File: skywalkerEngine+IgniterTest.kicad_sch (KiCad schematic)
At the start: 45 parts

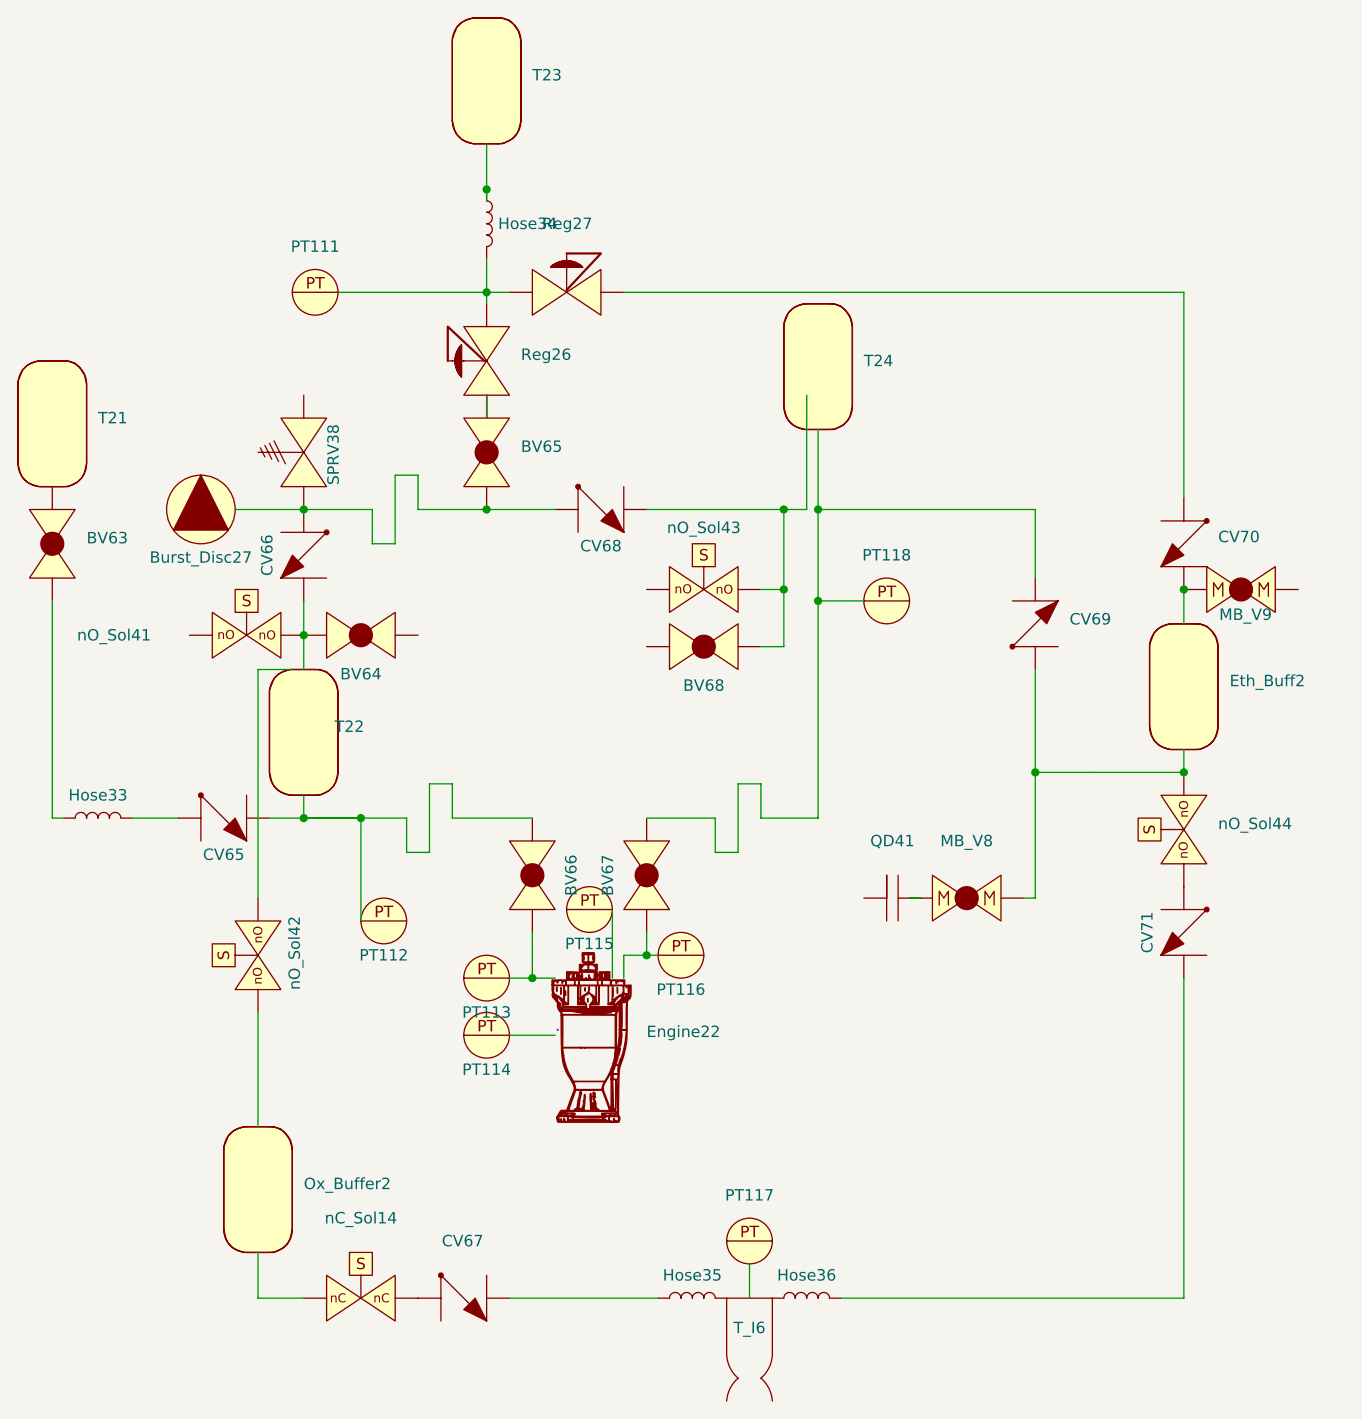
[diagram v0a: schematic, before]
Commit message: j0
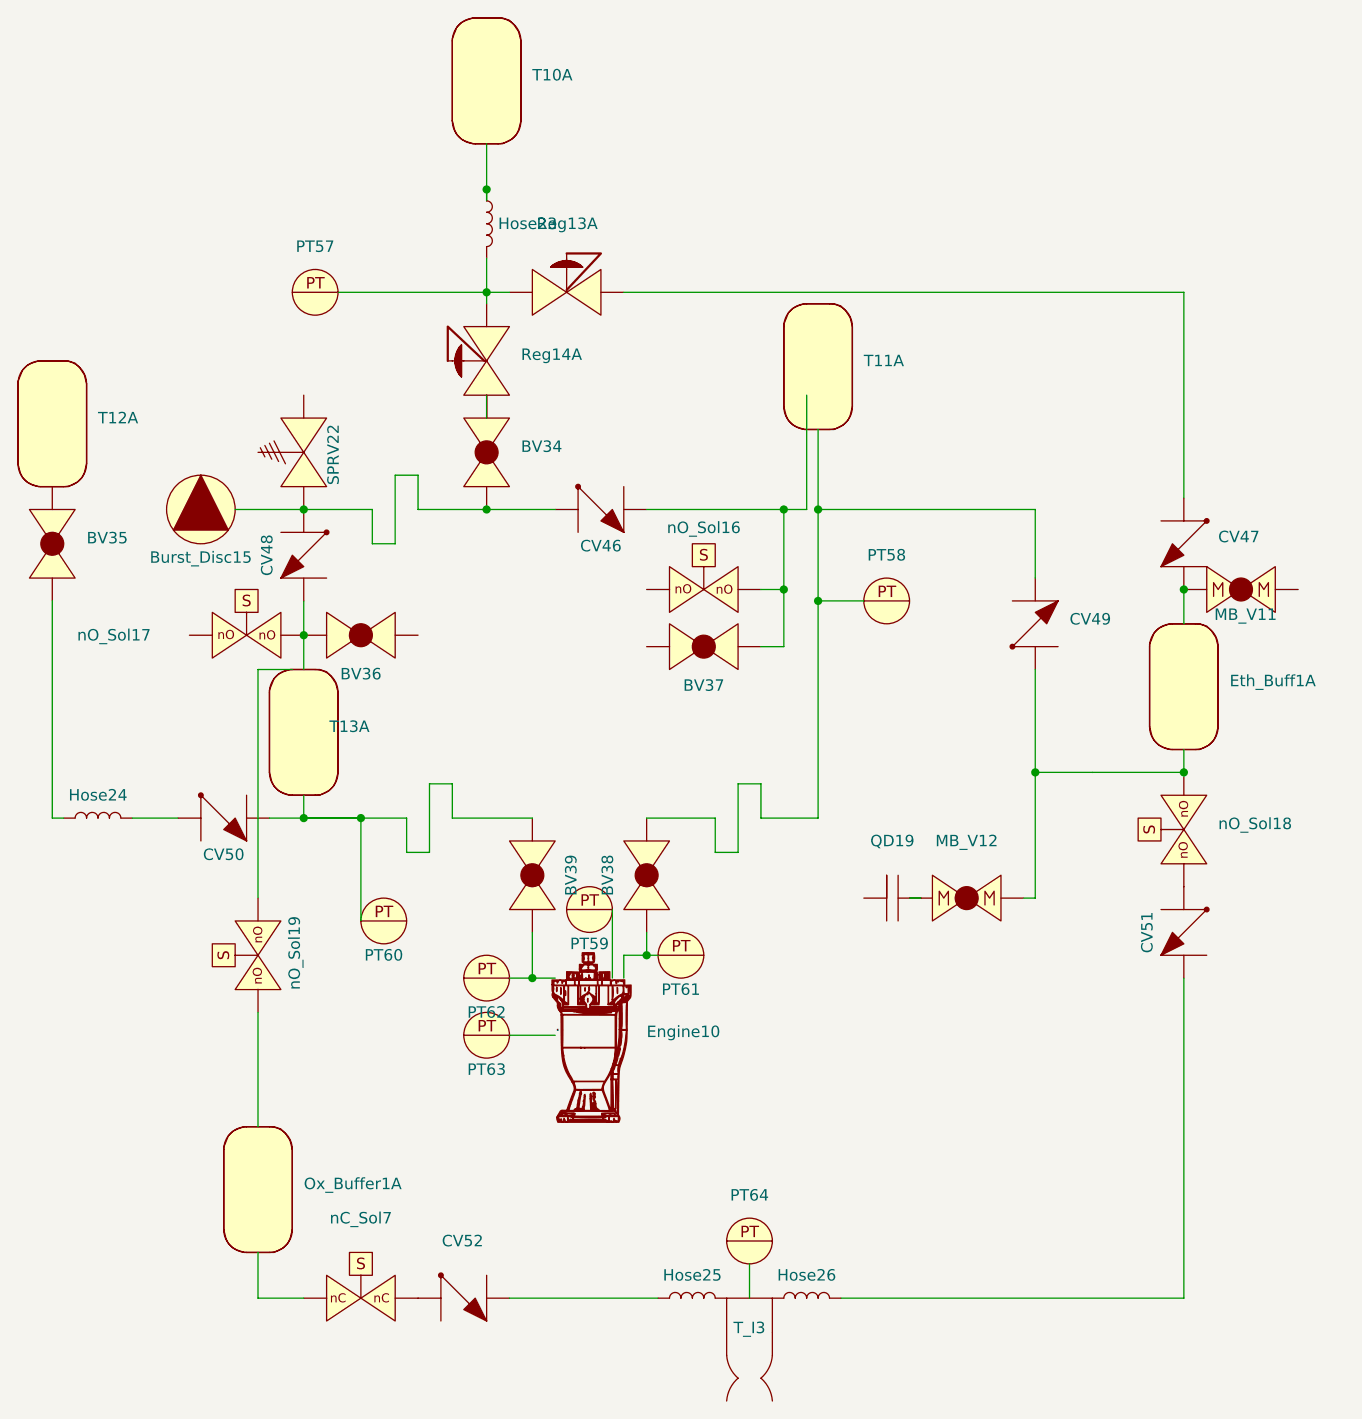
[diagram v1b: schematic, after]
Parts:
- renumbered BV65 to BV34, BV63 to BV35, BV64 to BV36, BV68 to BV37, BV67 to BV38, BV66 to BV39, Burst_Disc27 to Burst_Disc15, CV68 to CV46, CV70 to CV47, CV66 to CV48, CV69 to CV49, CV65 to CV50, CV71 to CV51, CV67 to CV52, Engine22 to Engine10, Eth_Buff2 to Eth_Buff1, Hose34 to Hose23, Hose33 to Hose24, Hose35 to Hose25, Hose36 to Hose26, MB_V9 to MB_V11, MB_V8 to MB_V12, Ox_Buffer2 to Ox_Buffer1, PT111 to PT57, PT118 to PT58, PT115 to PT59, PT112 to PT60, PT116 to PT61, PT113 to PT62, PT114 to PT63, PT117 to PT64, QD41 to QD19, Reg27 to Reg13, Reg26 to Reg14, SPRV38 to SPRV22, T23 to T10, T24 to T11, T21 to T12, T22 to T13, T_I6 to T_I3, nC_Sol14 to nC_Sol7, nO_Sol43 to nO_Sol16, nO_Sol41 to nO_Sol17, nO_Sol44 to nO_Sol18, nO_Sol42 to nO_Sol19
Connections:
- net at Engine10.: now also BV39., PT62.
- net at nC_Sol7.: now also Ox_Buffer1.; no longer CV52.
- net at Ox_Buffer1.: now also nO_Sol19.; no longer nC_Sol7.
- net at T10.: now also Hose23.1
- net at BV36.: now also CV48., T13., nO_Sol17.
- net at T12.: now also BV35.
- net at BV35.: now also Hose24.1; no longer T12.
- net at QD19.: now also MB_V12.
- net at BV37.: now also CV46., nO_Sol16.
- new net: CV49., Eth_Buff1., MB_V12., nO_Sol18.
- new net: BV38., CV49., PT58., T11.
- new net: BV38., Engine10., PT61.
- new net: CV47., Eth_Buff1., MB_V11.
- new net: CV52., nC_Sol7.
- new net: BV39., CV50., PT60., T13.
- new net: BV34., Burst_Disc15., CV46., CV48., SPRV22.
- now unconnected: Burst_Disc15., MB_V11., PT58., PT60., PT61., PT62., SPRV22., T11., nO_Sol16., nO_Sol17.

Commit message: more silwood stuff
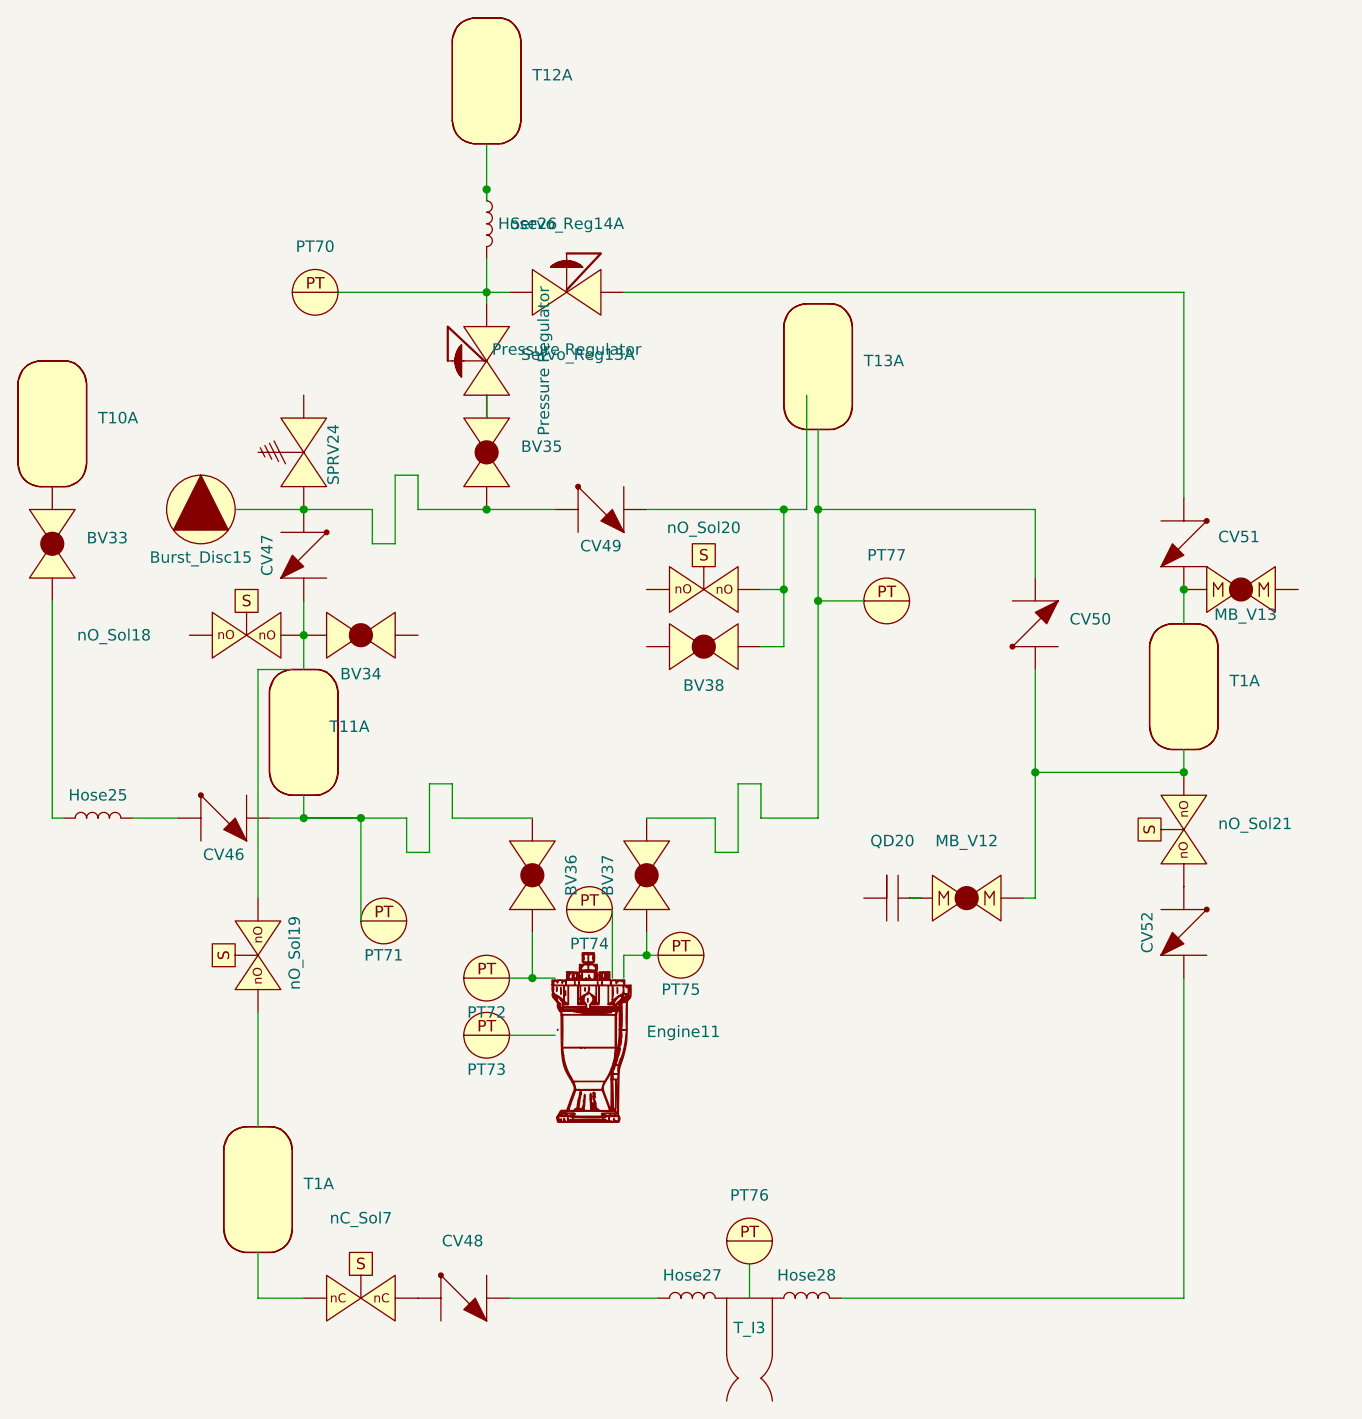
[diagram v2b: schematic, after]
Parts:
- renumbered BV35 to BV33, BV36 to BV34, BV34 to BV35, BV39 to BV36, BV38 to BV37, BV37 to BV38, CV50 to CV46, CV48 to CV47, CV52 to CV48, CV46 to CV49, CV49 to CV50, CV47 to CV51, CV51 to CV52, Engine10 to Engine11, Hose24 to Hose25, Hose23 to Hose26, Hose25 to Hose27, Hose26 to Hose28, MB_V11 to MB_V13, PT57 to PT70, PT60 to PT71, PT62 to PT72, PT63 to PT73, PT59 to PT74, PT61 to PT75, PT64 to PT76, PT58 to PT77, QD19 to QD20, SPRV22 to SPRV24, Reg14 to Servo_Reg13, Reg13 to Servo_Reg14, Eth_Buff1 to T1, Ox_Buffer1 to T1, T12 to T10, T13 to T11, T10 to T12, T11 to T13, nO_Sol17 to nO_Sol18, nO_Sol16 to nO_Sol20, nO_Sol18 to nO_Sol21
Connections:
- net at Engine11.: now also BV36., PT72.
- net at nC_Sol7.: now also T1.; no longer CV48.
- net at T1.: now also nO_Sol19.; no longer nC_Sol7.
- net at T12.: now also Hose26.1
- net at BV34.: now also CV47., T11., nO_Sol18.
- net at T10.: now also BV33.
- net at BV33.: now also Hose25.1; no longer T10.
- net at QD20.: now also MB_V12.
- net at BV38.: now also CV49., nO_Sol20.
- new net: CV50., MB_V12., T1., nO_Sol21.
- new net: BV37., CV50., PT77., T13.
- new net: BV37., Engine11., PT75.
- new net: CV51., MB_V13., T1.
- new net: CV48., nC_Sol7.
- new net: BV36., CV46., PT71., T11.
- new net: BV35., Burst_Disc15., CV47., CV49., SPRV24.
- now unconnected: Burst_Disc15., MB_V13., PT71., PT72., PT75., PT77., SPRV24., T13., nO_Sol18., nO_Sol20.

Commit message: Formatiing
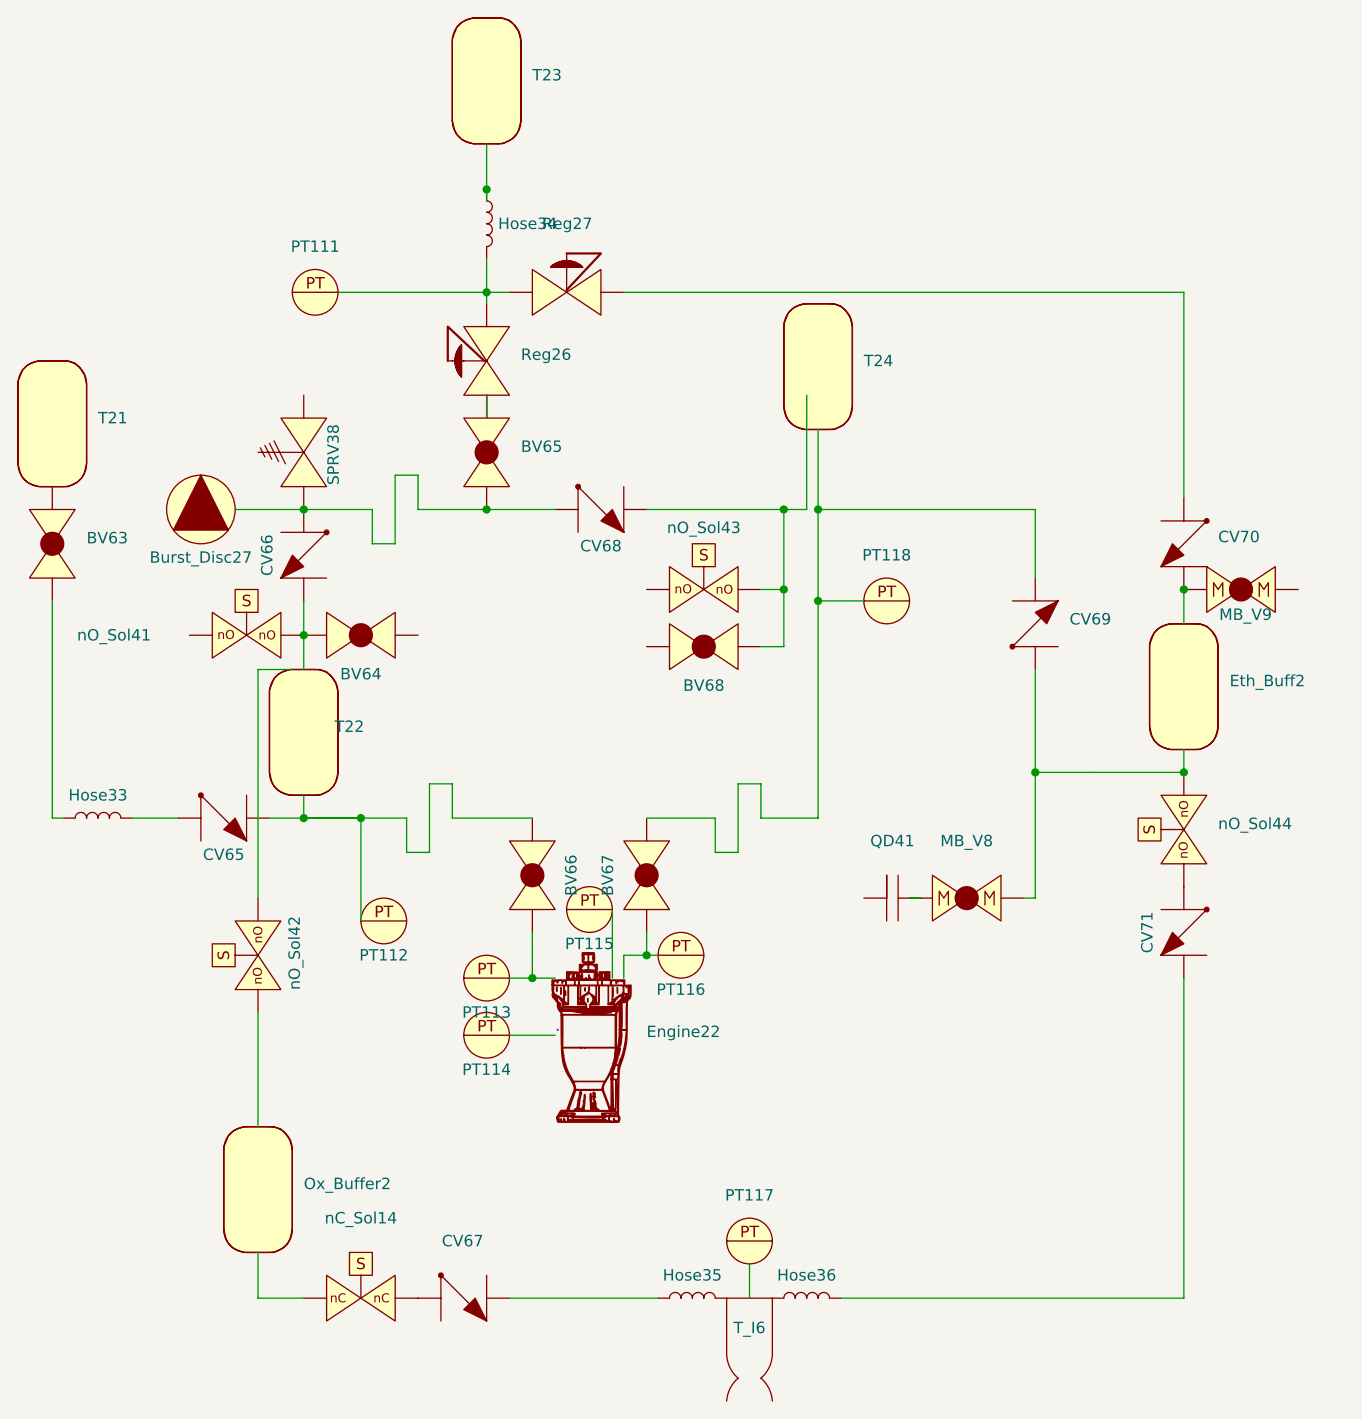
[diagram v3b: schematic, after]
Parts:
- renumbered BV33 to BV63, BV34 to BV64, BV35 to BV65, BV36 to BV66, BV37 to BV67, BV38 to BV68, Burst_Disc15 to Burst_Disc27, CV46 to CV65, CV47 to CV66, CV48 to CV67, CV49 to CV68, CV50 to CV69, CV51 to CV70, CV52 to CV71, Engine11 to Engine22, T1 to Eth_Buff2, Hose25 to Hose33, Hose26 to Hose34, Hose27 to Hose35, Hose28 to Hose36, MB_V12 to MB_V8, MB_V13 to MB_V9, T1 to Ox_Buffer2, PT70 to PT111, PT71 to PT112, PT72 to PT113, PT73 to PT114, PT74 to PT115, PT75 to PT116, PT76 to PT117, PT77 to PT118, QD20 to QD41, Servo_Reg13 to Reg26, Servo_Reg14 to Reg27, SPRV24 to SPRV38, T10 to T21, T11 to T22, T12 to T23, T13 to T24, T_I3 to T_I6, nC_Sol7 to nC_Sol14, nO_Sol18 to nO_Sol41, nO_Sol19 to nO_Sol42, nO_Sol20 to nO_Sol43, nO_Sol21 to nO_Sol44
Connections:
- net at Engine22.: now also BV66., PT113.
- net at nC_Sol14.: now also Ox_Buffer2.; no longer CV67.
- net at Ox_Buffer2.: now also nO_Sol42.; no longer nC_Sol14.
- net at T23.: now also Hose34.1
- net at BV64.: now also CV66., T22., nO_Sol41.
- net at T21.: now also BV63.
- net at BV63.: now also Hose33.1; no longer T21.
- net at QD41.: now also MB_V8.
- net at BV68.: now also CV68., nO_Sol43.
- new net: CV69., Eth_Buff2., MB_V8., nO_Sol44.
- new net: BV67., CV69., PT118., T24.
- new net: BV67., Engine22., PT116.
- new net: CV70., Eth_Buff2., MB_V9.
- new net: CV67., nC_Sol14.
- new net: BV66., CV65., PT112., T22.
- new net: BV65., Burst_Disc27., CV66., CV68., SPRV38.
- now unconnected: Burst_Disc27., MB_V9., PT112., PT113., PT116., PT118., SPRV38., T24., nO_Sol41., nO_Sol43.
